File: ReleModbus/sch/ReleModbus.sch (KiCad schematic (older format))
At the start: 47 parts, among them J1 PWR, J2 ICSP, J3 I2C, J4 DB9_FEMALE, J5 COMUM, J6 N_ABERTO, J7 N_FECHADO, Q1 BC817, Q2 BC817, U1 ATMEGA328P-AU, U2 LM7805CT, U3 MAX232, Y1 16MHz

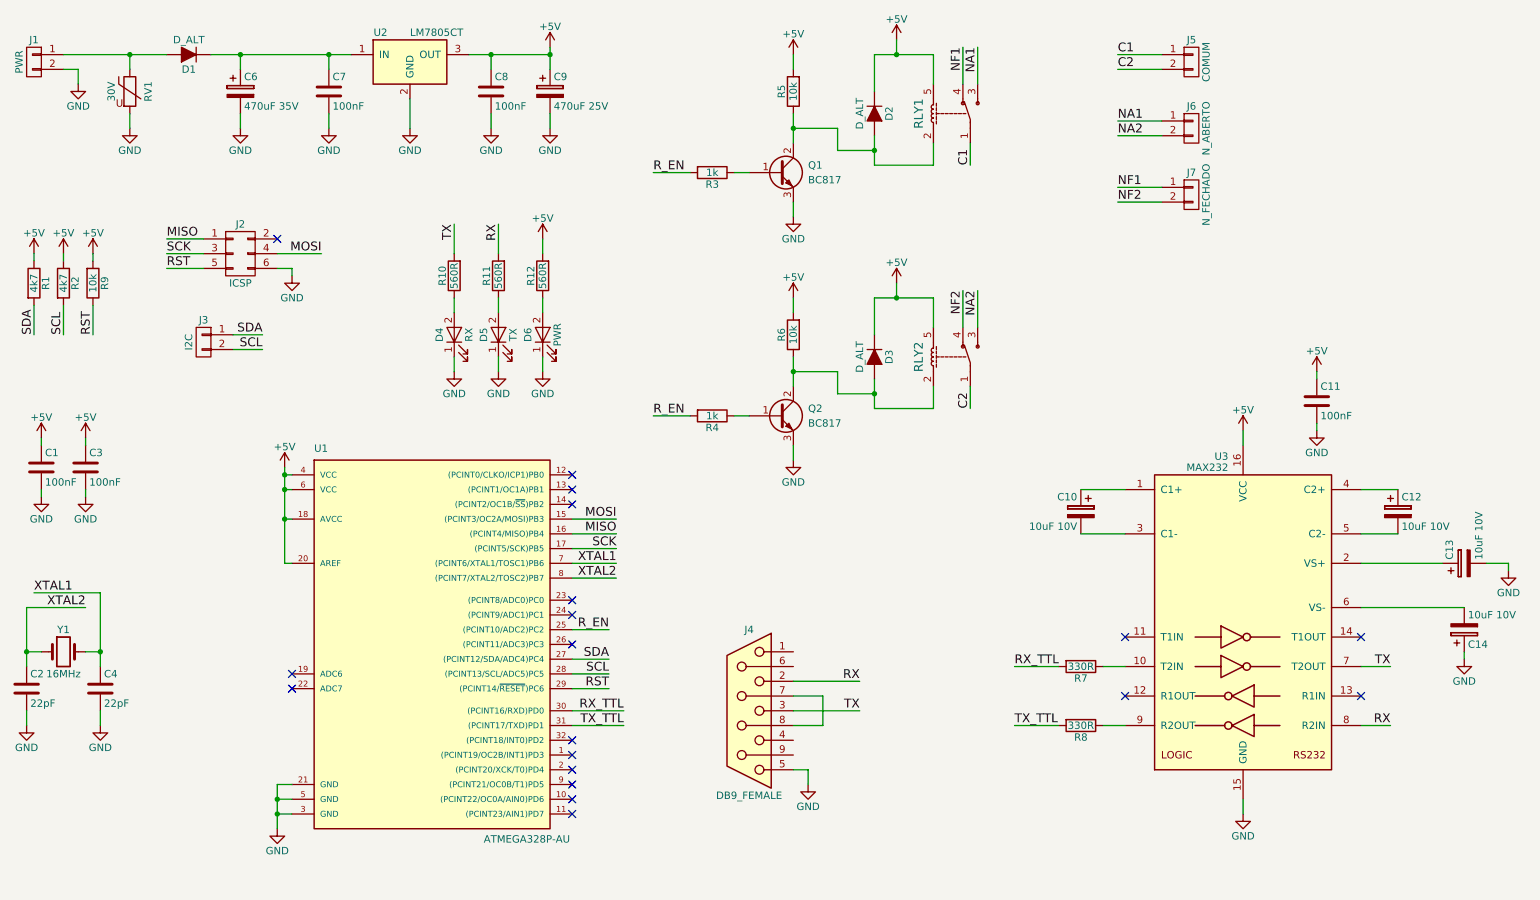
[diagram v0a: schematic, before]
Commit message: Signed-off-by: cuki2 <mauricio@krebs.com.br>
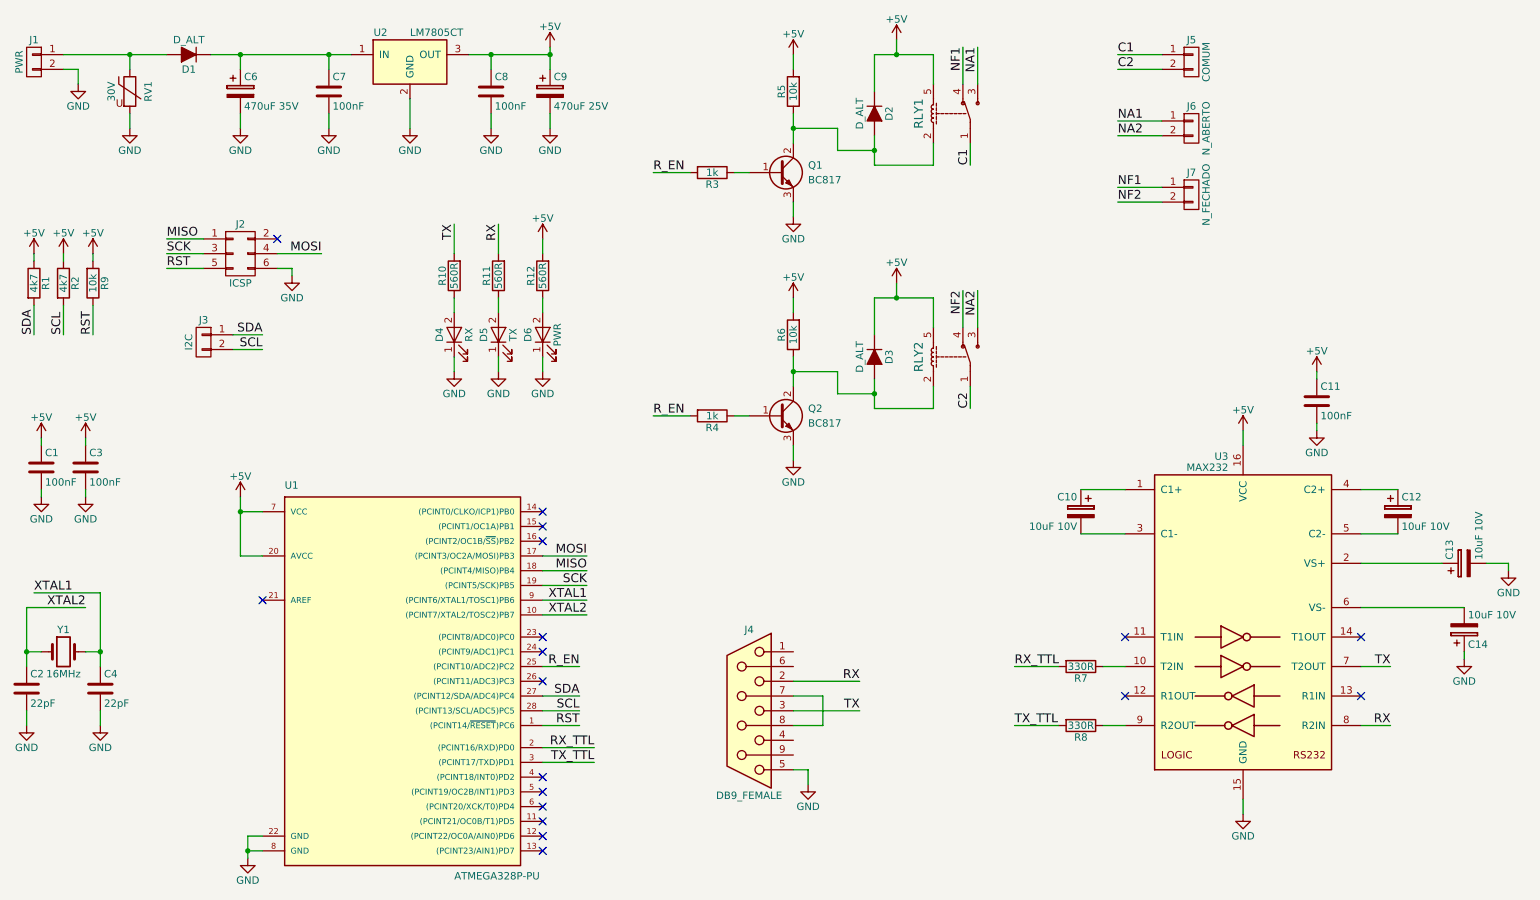
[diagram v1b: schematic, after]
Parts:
- removed U1: ATMEGA328P-AU, w_smd_lqfp:lqfp32, symbol ATMEGA328P-AU
- added U1: ATMEGA328P-PU, w_pth_circuits:dil_28-300, symbol ATMEGA328P-PU
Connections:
- net +5V: now also U1.20 (AVCC), U1.7 (VCC)
- net GND: now also U1.22 (GND), U1.8 (GND)
- net MISO: now also U1.18 ((PCINT4/MISO)PB4)
- net MOSI: now also U1.17 ((PCINT3/OC2A/MOSI)PB3)
- net RST: now also U1.1 ((PCINT14/~RESET~)PC6)
- net RX_TTL: now also U1.2 ((PCINT16/RXD)PD0)
- net R_EN: now also U1.25 ((PCINT10/ADC2)PC2)
- net SCK: now also U1.19 ((PCINT5/SCK)PB5)
- net SCL: now also U1.28 ((PCINT13/SCL/ADC5)PC5)
- net SDA: now also U1.27 ((PCINT12/SDA/ADC4)PC4)
- net TX_TTL: now also U1.3 ((PCINT17/TXD)PD1)
- net XTAL1: now also U1.9 ((PCINT6/XTAL1/TOSC1)PB6)
- net XTAL2: now also U1.10 ((PCINT7/XTAL2/TOSC2)PB7)
- no-connect marks 19 -> 18
